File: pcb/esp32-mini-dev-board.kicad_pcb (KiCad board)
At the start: 2 copper layers, 39.9 x 52 mm, 11 parts, among them J1 USB_C_Receptacle_USB2.0_16P, U1 USBLC6-2SC6, U2 AP2112K-3.3, U3 ESP32-C3-WROOM-02

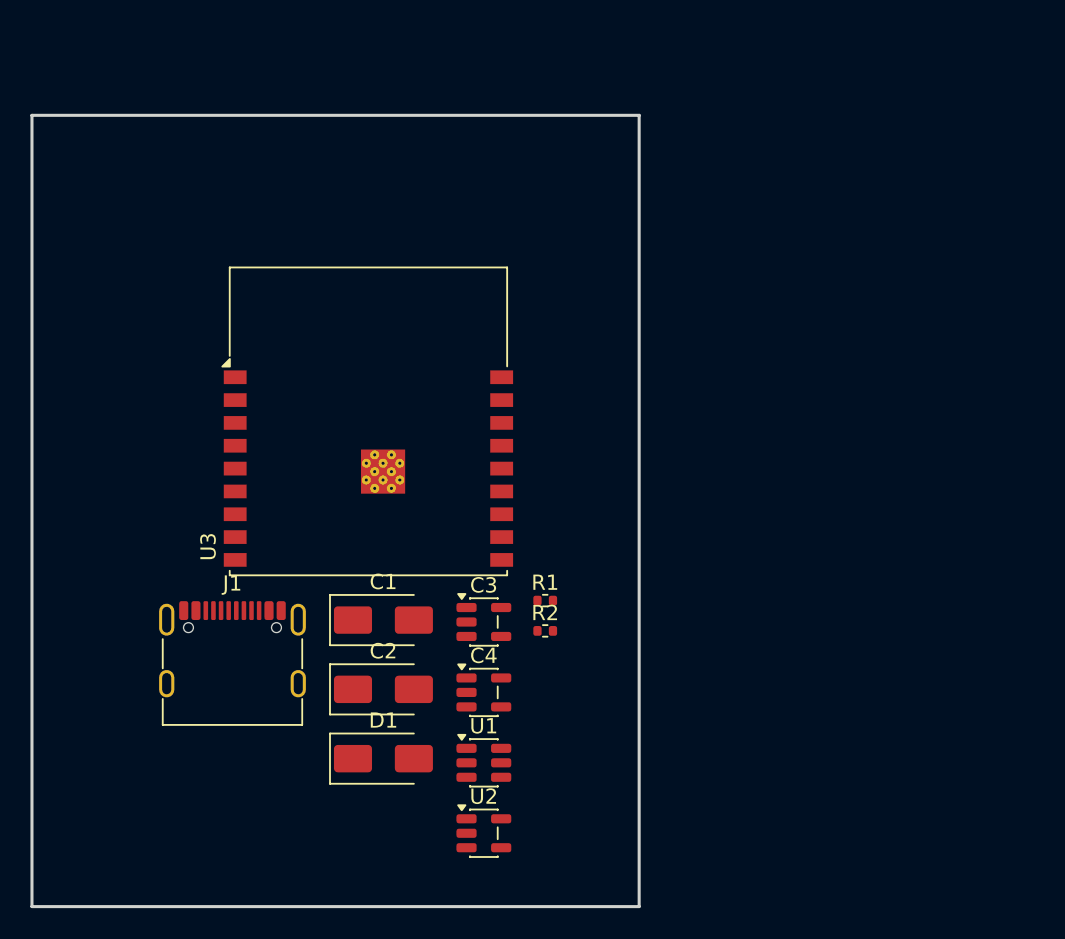
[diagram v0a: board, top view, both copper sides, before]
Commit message: feat(lay): add first placement of all parts
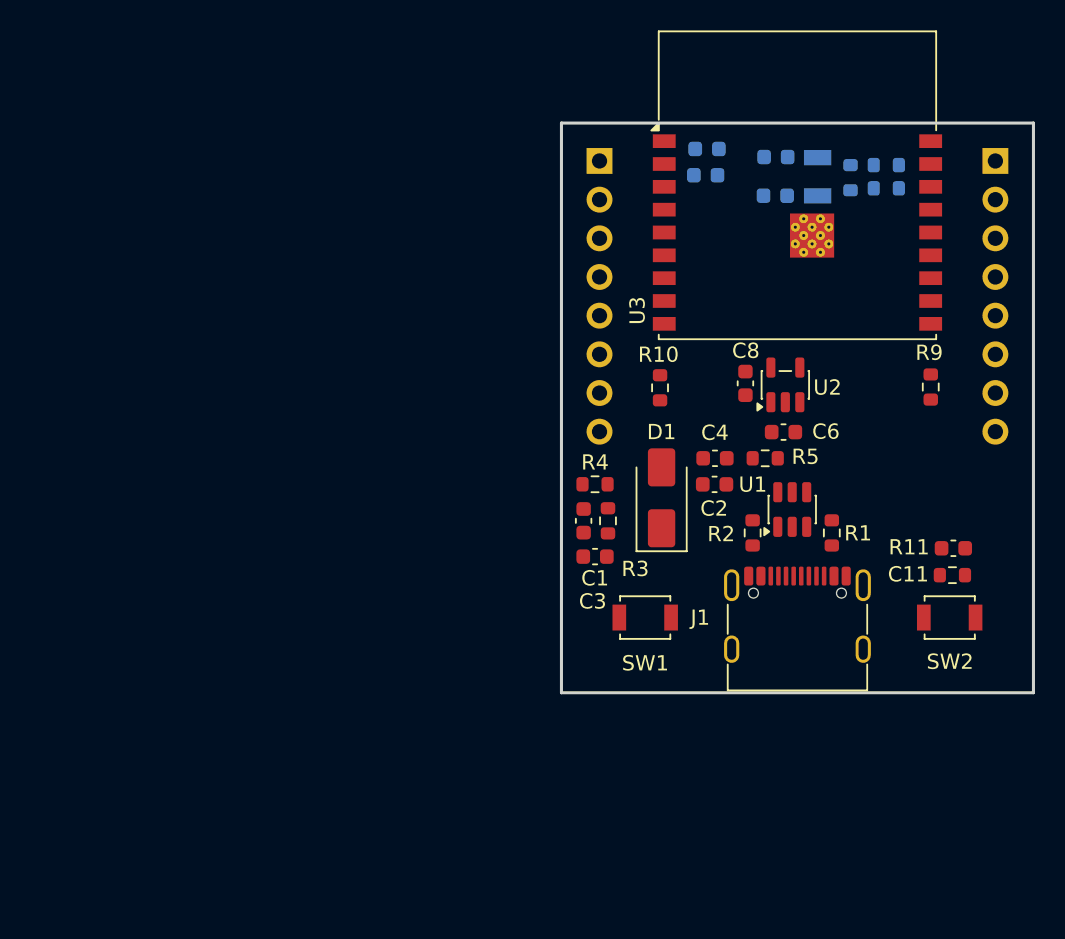
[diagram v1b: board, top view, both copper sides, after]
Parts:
- added C10: 100n, Capacitor_SMD:C_0603_1608Metric, B.Cu at (157.0, 100.9)
- added C11: C, Capacitor_SMD:C_0603_1608Metric, F.Cu at (173.2, 125.4)
- added C5: C, Capacitor_SMD:C_0603_1608Metric, B.Cu at (161.6, 99.7)
- added C6: 4u7, Capacitor_SMD:C_0603_1608Metric, F.Cu at (162.1, 117.8)
- added C7: C, Capacitor_SMD:C_0603_1608Metric, B.Cu at (161.5, 102.3)
- added C8: 4u7, Capacitor_SMD:C_0603_1608Metric, F.Cu at (159.6, 114.6)
- added C9: 4u7, Capacitor_SMD:C_0603_1608Metric, B.Cu at (157.1, 99.2)
- added J2: Conn_01x08_Pin, Connector_PinHeader_2.54mm:PinHeader_1x08_P2.54mm_Vertical, B.Cu at (150.0, 100.0)
- added J3: Conn_01x08_Pin, Connector_PinHeader_2.54mm:PinHeader_1x08_P2.54mm_Vertical, B.Cu at (176.0, 100.0)
- added R10: R, Resistor_SMD:R_0603_1608Metric, F.Cu at (154.0, 114.9)
- added R11: R, Resistor_SMD:R_0603_1608Metric, F.Cu at (173.2, 127.2)
- added R3: R, Resistor_SMD:R_0603_1608Metric, F.Cu at (150.6, 123.6)
- added R4: R, Resistor_SMD:R_0603_1608Metric, F.Cu at (149.7, 121.2)
- added R5: 0R, Resistor_SMD:R_0603_1608Metric, F.Cu at (160.9, 119.5)
- added R6: 0R, Resistor_SMD:R_0603_1608Metric, B.Cu at (168.8, 100.3)
- added R7: R, Resistor_SMD:R_0603_1608Metric, B.Cu at (166.5, 101.1)
- added R8: 0R, Resistor_SMD:R_0603_1608Metric, B.Cu at (168.8, 101.8)
- added R9: R, Resistor_SMD:R_0603_1608Metric, F.Cu at (171.8, 114.8)
- added SW1: SW_Push, Button_Switch_SMD:SW_SPST_B3U-1000P, F.Cu at (153.0, 130.0)
- added SW2: SW_Push, Button_Switch_SMD:SW_SPST_B3U-1000P, F.Cu at (173.0, 130.0)
- added Y1: Crystal, Crystal:Crystal_SMD_3215-2Pin_3.2x1.5mm, B.Cu at (164.3, 101.0)
- C1: value 4u7 -> C; footprint Diode_SMD:D_SMA -> Capacitor_SMD:C_0603_1608Metric
- C2: footprint Diode_SMD:D_SMA -> Capacitor_SMD:C_0603_1608Metric
- C3: value 4u7 -> C; footprint Package_TO_SOT_SMD:SOT-23-5 -> Capacitor_SMD:C_0603_1608Metric
- C4: footprint Package_TO_SOT_SMD:SOT-23-5 -> Capacitor_SMD:C_0603_1608Metric
- R1, R2: footprint Resistor_SMD:R_0402_1005Metric -> Resistor_SMD:R_0603_1608Metric
- moved J1 37.2 mm to (163.0, 131.0)
- moved U2 35.5 mm to (162.2, 114.7), turned to 90 degrees
- moved U3 32.2 mm to (163.0, 104.7)
- moved U1 26.2 mm to (162.7, 122.9), turned to 90 degrees
- moved C2 25.6 mm to (157.6, 121.2), turned to 180 degrees
- moved D1 25.0 mm to (154.1, 122.1), turned to 90 degrees
- moved C4 21.6 mm to (157.6, 119.5), turned to 180 degrees
- moved R1 19.3 mm to (165.3, 124.4), turned to 90 degrees
- moved R2 15.1 mm to (160.1, 124.4), turned to 90 degrees
- moved C1 14.5 mm to (149.7, 126.0), turned to 180 degrees
- moved C3 9.33 mm to (149.0, 123.6), turned to -90 degrees
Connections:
- net Net-(U2-EN) renamed +5V
- C1 pad 1: Net-(D1-A1) -> Net-(C1-Pad1)
- C2 pad 1: Net-(C2-Pad1) -> Net-(D1-A1)
- C3 pad 1: Net-(U2-VOUT) -> /CIRCUIT DESIGN/EN_RST
- U1 pad 4: USB_D+ -> /CIRCUIT DESIGN/USB_D+
- U1 pad 6: USB_D- -> /CIRCUIT DESIGN/USB_D-
- U2 pad 5: Net-(U2-VOUT) -> +3V3
- U3 pad 1: unconnected-(U3-3V3-Pad1) -> +3V3
- U3 pad 10: unconnected-(U3-IO10-Pad10) -> /CIRCUIT DESIGN/IO10
- U3 pad 11: unconnected-(U3-IO20/RXD-Pad11) -> /CIRCUIT DESIGN/RXD
- U3 pad 12: unconnected-(U3-IO21/TXD-Pad12) -> /CIRCUIT DESIGN/TXD
- U3 pad 13: unconnected-(U3-IO18-Pad13) -> /CIRCUIT DESIGN/USB_D-
- U3 pad 14: unconnected-(U3-IO19-Pad14) -> /CIRCUIT DESIGN/USB_D+
- U3 pad 15: unconnected-(U3-IO3-Pad15) -> /CIRCUIT DESIGN/IO3
- U3 pad 16: unconnected-(U3-IO2-Pad16) -> Net-(U3-IO2)
- U3 pad 17: unconnected-(U3-IO1-Pad17) -> /CIRCUIT DESIGN/XTAL_32K_N
- U3 pad 18: unconnected-(U3-IO0-Pad18) -> /CIRCUIT DESIGN/XTAL_32K_P
- U3 pad 19: Net-(U3-GND-Pad19) -> GND
- U3 pad 2: unconnected-(U3-EN-Pad2) -> /CIRCUIT DESIGN/EN
- U3 pad 3: unconnected-(U3-IO4-Pad3) -> /CIRCUIT DESIGN/IO4
- U3 pad 4: unconnected-(U3-IO5-Pad4) -> /CIRCUIT DESIGN/IO5
- U3 pad 5: unconnected-(U3-IO6-Pad5) -> /CIRCUIT DESIGN/IO6
- U3 pad 6: unconnected-(U3-IO7-Pad6) -> /CIRCUIT DESIGN/IO7
- U3 pad 7: unconnected-(U3-IO8-Pad7) -> Net-(U3-IO8)
- U3 pad 8: unconnected-(U3-IO9-Pad8) -> /CIRCUIT DESIGN/BOOT
- U3 pad 9: Net-(U3-GND-Pad19) -> GND
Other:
- board size 39.9 x 52 mm -> 31 x 37.4 mm
